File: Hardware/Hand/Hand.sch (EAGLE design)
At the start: 27 parts, among them T1 2N3904, T2 2N3904, T3 2N3904

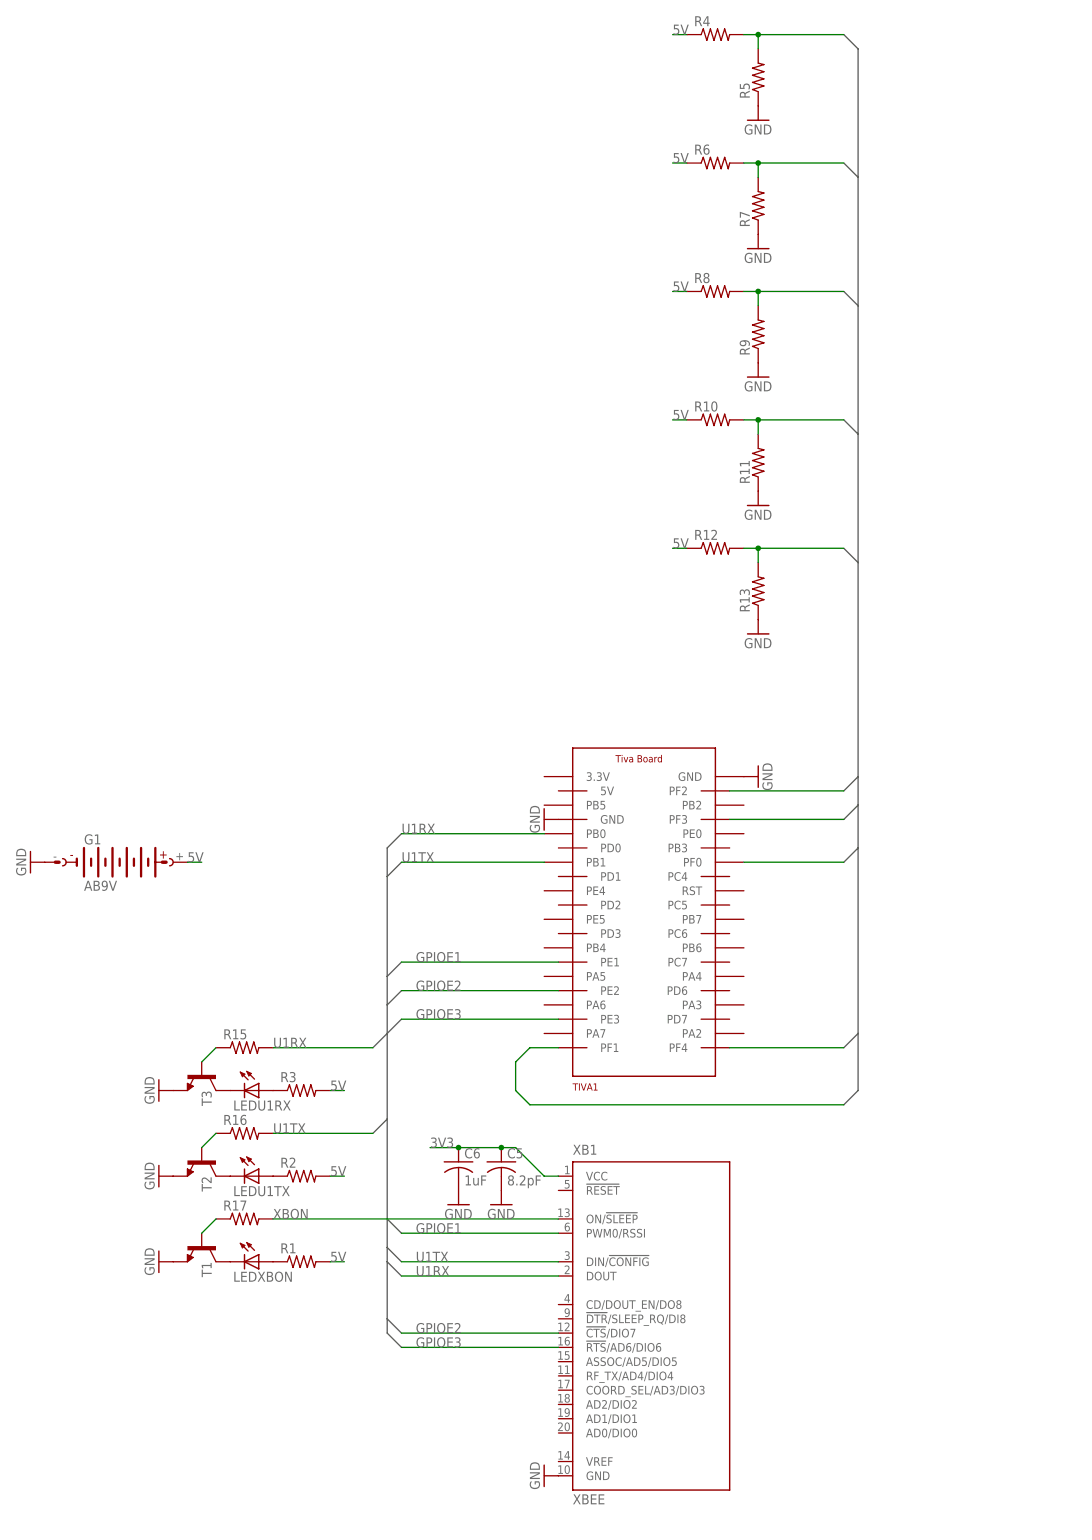
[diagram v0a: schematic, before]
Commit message: Hand PCB Rev0 complete.
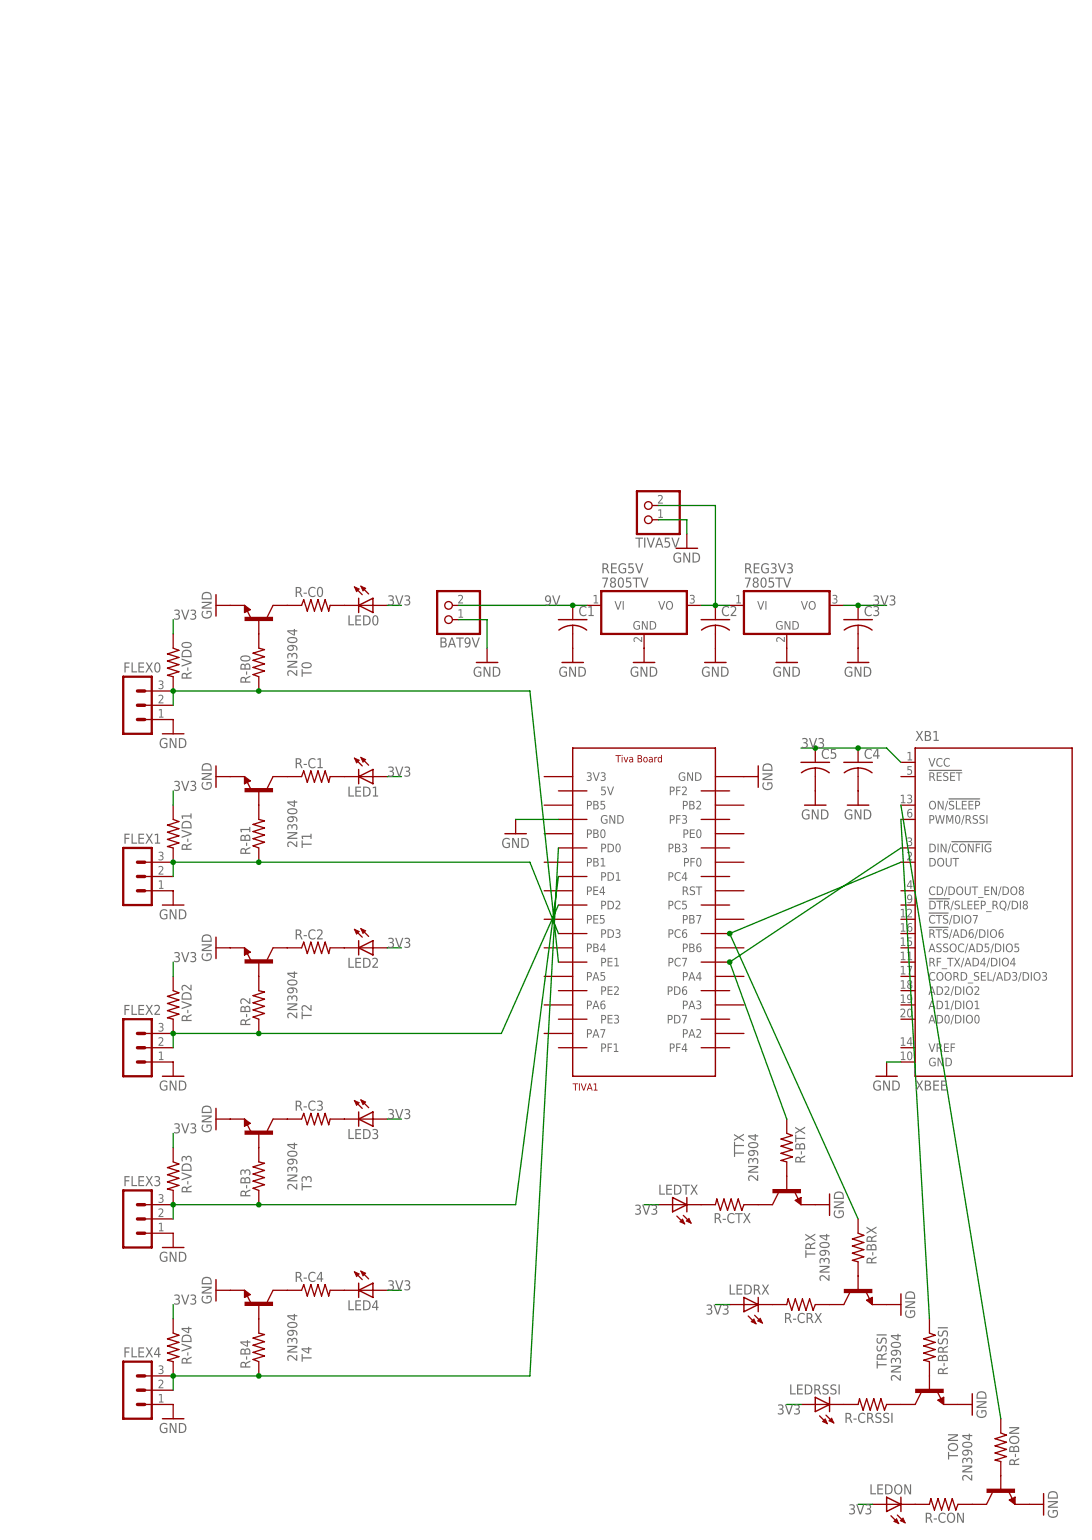
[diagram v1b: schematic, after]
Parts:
- removed C6: 1uF, rcl:C-US025-025X050
- removed G1: AB9V, battery:AB9V
- removed LEDU1RX, LEDU1TX, LEDXBON: (no value), led:LED5MM
- removed R1, R10, R11, R12, R13, R15, R16, R17, R2, R3, R4, R5, R6, R7, R8, R9: (no value), rcl:R-US_0207/7
- added BAT9V, TIVA5V: (no value), pinhead:PINHD-1X2
- added C1, C2, C3, C4: (no value), rcl:C-US025-025X050
- added FLEX0, FLEX1, FLEX2, FLEX3, FLEX4: (no value), con-lstb:MA03-1
- added LED0, LED1, LED2, LED3, LED4, LEDON, LEDRSSI, LEDRX, LEDTX: (no value), led:LED5MM
- added R-B0, R-B1, R-B2, R-B3, R-B4, R-BON, R-BRSSI, R-BRX, R-BTX, R-C0, R-C1, R-C2, R-C3, R-C4, R-CON, R-CRSSI, R-CRX, R-CTX, R-VD0, R-VD1, R-VD2, R-VD3, R-VD4: (no value), resistor:R-US_0204/7
- added REG3V3, REG5V: 7805TV, linear:7805TV
- added T0, T4, TON, TRSSI, TRX, TTX: 2N3904, transistor:2N3904
- C5: value 8.2pF -> (none)
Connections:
- removed net B$1: R10.2, R11.2, R12.2, R13.2, R4.2, R5.2, R6.2, R7.2, R8.2, R9.2, TIVA1.PF0, TIVA1.PF1, TIVA1.PF2, TIVA1.PF3, TIVA1.PF4
- removed net GPIOE1: TIVA1.PE1, XB1.PWM0/RSSI
- removed net GPIOE2: TIVA1.PE2, XB1.!CTS!/DIO7
- removed net GPIOE3: TIVA1.PE3, XB1.!RTS!/AD6/DIO6
- removed net U1RX: R15.2, TIVA1.PB0, XB1.DOUT
- removed net U1TX: R16.2, TIVA1.PB1, XB1.DIN/!CONFIG
- removed net XBON: R17.2, XB1.ON/!SLEEP
- new net 9V: BAT9V.2, C1.1, REG5V.VI
- new net N$10: R-B1.2, T1.B
- new net N$11: LED4.C, R-C4.2
- new net N$12: LED2.C, R-C2.2
- new net N$13: FLEX2.2, FLEX2.3, R-B2.1, R-VD2.2, TIVA1.PD2
- new net N$14: R-B2.2, T2.B
- new net N$15: R-C0.1, T0.C
- new net N$16: LED0.C, R-C0.2
- new net N$17: FLEX3.2, FLEX3.3, R-B3.1, R-VD3.2, TIVA1.PD1
- new net N$18: R-B3.2, T3.B
- new net N$19: R-BTX.1, TIVA1.PC7, XB1.DIN/!CONFIG
- new net N$20: R-BRX.1, TIVA1.PC6, XB1.DOUT
- new net N$21: FLEX4.2, FLEX4.3, R-B4.1, R-VD4.2, TIVA1.PD0
- new net N$22: R-B4.2, T4.B
- new net N$23: R-BTX.2, TTX.B
- new net N$24: R-CTX.1, TTX.C
- new net N$25: LEDTX.C, R-CTX.2
- new net N$26: R-BRX.2, TRX.B
- new net N$27: R-CRX.1, TRX.C
- new net N$31: R-BRSSI.2, TRSSI.B
- new net N$32: R-CRSSI.1, TRSSI.C
- new net N$33: LEDRSSI.C, R-CRSSI.2
- new net N$34: R-BON.2, TON.B
- new net N$35: R-CON.1, TON.C
- new net N$36: LEDON.C, R-CON.2
- new net N$7: LED3.C, R-C3.2
- new net N$8: R-C4.1, T4.C
- new net N$9: FLEX1.2, FLEX1.3, R-B1.1, R-VD1.2, TIVA1.PD3
- net 3V3: now also C3.1, C4.1, LED0.A, LED1.A, LED2.A, LED3.A, LED4.A, LEDON.A, LEDRSSI.A, LEDRX.A, LEDTX.A, R-VD0.1, R-VD1.1, R-VD2.1, R-VD3.1, R-VD4.1, REG3V3.VO; no longer C6.1
- net 5V: now also C2.1, REG3V3.VI, REG5V.VO, TIVA5V.2; no longer R1.2, R10.1, R12.1, R2.2, R3.2, R4.1, R6.1, R8.1
- net GND: now also BAT9V.1, C1.2, C2.2, C3.2, C4.2, FLEX0.1, FLEX1.1, FLEX2.1, FLEX3.1, FLEX4.1, REG3V3.GND, REG5V.GND, T0.E, T4.E, TIVA5V.1, TON.E, TRSSI.E, TRX.E, TTX.E; no longer C6.2, G1.-, R11.1, R13.1, R5.1, R7.1, R9.1
- net N$1: now also FLEX0.2, FLEX0.3, R-B0.1, R-VD0.2, TIVA1.PE1; no longer LEDXBON.C, T1.C
- net N$2: now also R-C1.1, T1.C; no longer LEDU1TX.C, T2.C
- net N$28: now also LEDRX.C, R-CRX.2; no longer R15.1, T3.B
- net N$29: now also R-BRSSI.1, XB1.PWM0/RSSI; no longer R16.1, T2.B
- net N$3: now also LED1.C, R-C1.2; no longer LEDU1TX.A, R2.1
- net N$30: now also R-BON.1, XB1.ON/!SLEEP; no longer R17.1, T1.B
- net N$4: now also R-C2.1, T2.C; no longer LEDXBON.A, R1.1
- net N$5: now also R-B0.2, T0.B; no longer LEDU1RX.C, T3.C
- net N$6: now also R-C3.1, T3.C; no longer LEDU1RX.A, R3.1
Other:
- moved on the sheet: C5, T1, T2, T3, XB1
